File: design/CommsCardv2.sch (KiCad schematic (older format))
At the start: 0 parts

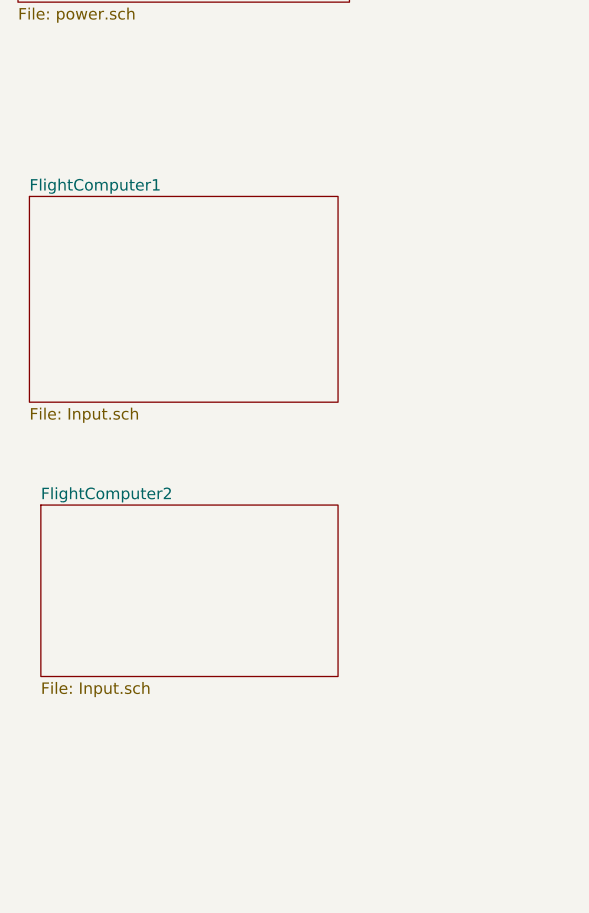
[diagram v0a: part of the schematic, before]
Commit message: Remove annotation
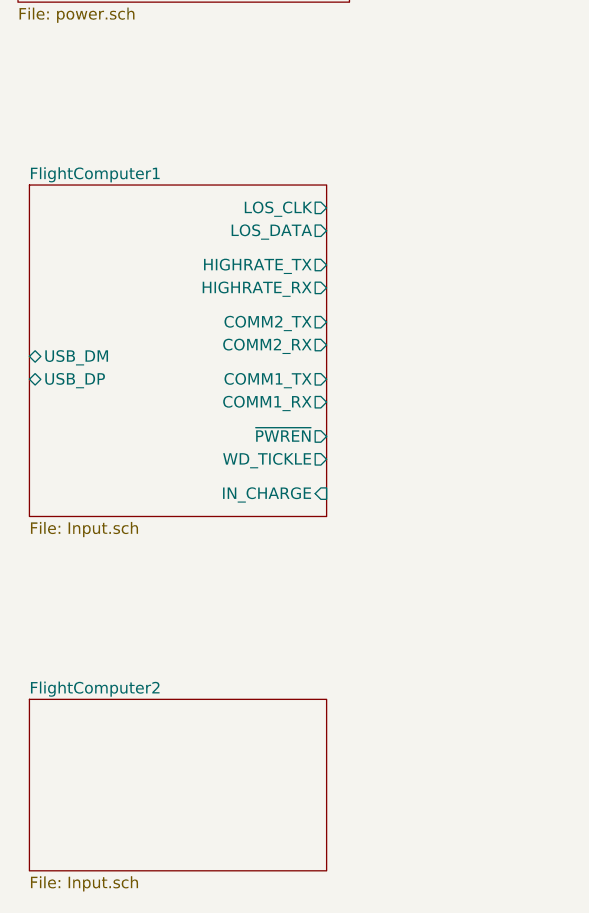
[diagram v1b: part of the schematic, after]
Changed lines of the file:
@@
 $EndSheet
 $Sheet
-S 2050 4150 1350 900
+S 2050 4100 1300 1450
 U 5A78E64E
 F0 "FlightComputer1" 50
 F1 "Input.sch" 50
+F2 "USB_DM" B L 2050 4850 50
+F3 "USB_DP" B L 2050 4950 50
+F4 "LOS_CLK" O R 3350 4200 50
+F5 "LOS_DATA" O R 3350 4300 50
+F6 "HIGHRATE_TX" O R 3350 4450 50
+F7 "HIGHRATE_RX" O R 3350 4550 50
+F8 "COMM2_TX" O R 3350 4700 50
+F9 "COMM2_RX" O R 3350 4800 50
+F10 "COMM1_TX" O R 3350 4950 50
+F11 "COMM1_RX" O R 3350 5050 50
+F12 "~PWREN" O R 3350 5200 50
+F13 "IN_CHARGE" I R 3350 5450 50
+F14 "WD_TICKLE" O R 3350 5300 50
 $EndSheet
 $Sheet
-S 2100 5500 1300 750
+S 2050 6350 1300 750
 U 5A78E661
 F0 "FlightComputer2" 50
